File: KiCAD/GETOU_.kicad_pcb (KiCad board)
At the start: 2 copper layers, 109.5 x 59.5 mm, 25 parts, among them U1 XIAO-RP2040-DIP

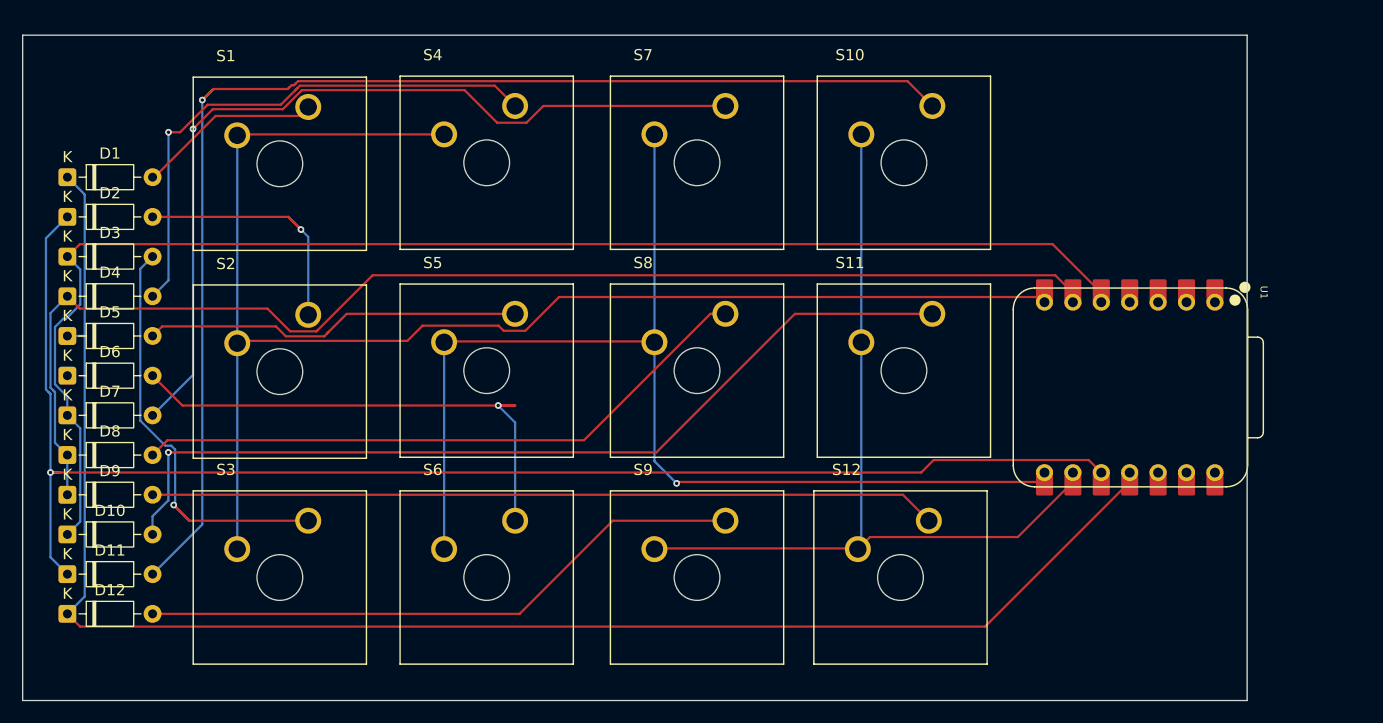
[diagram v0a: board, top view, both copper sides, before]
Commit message: Add stuff
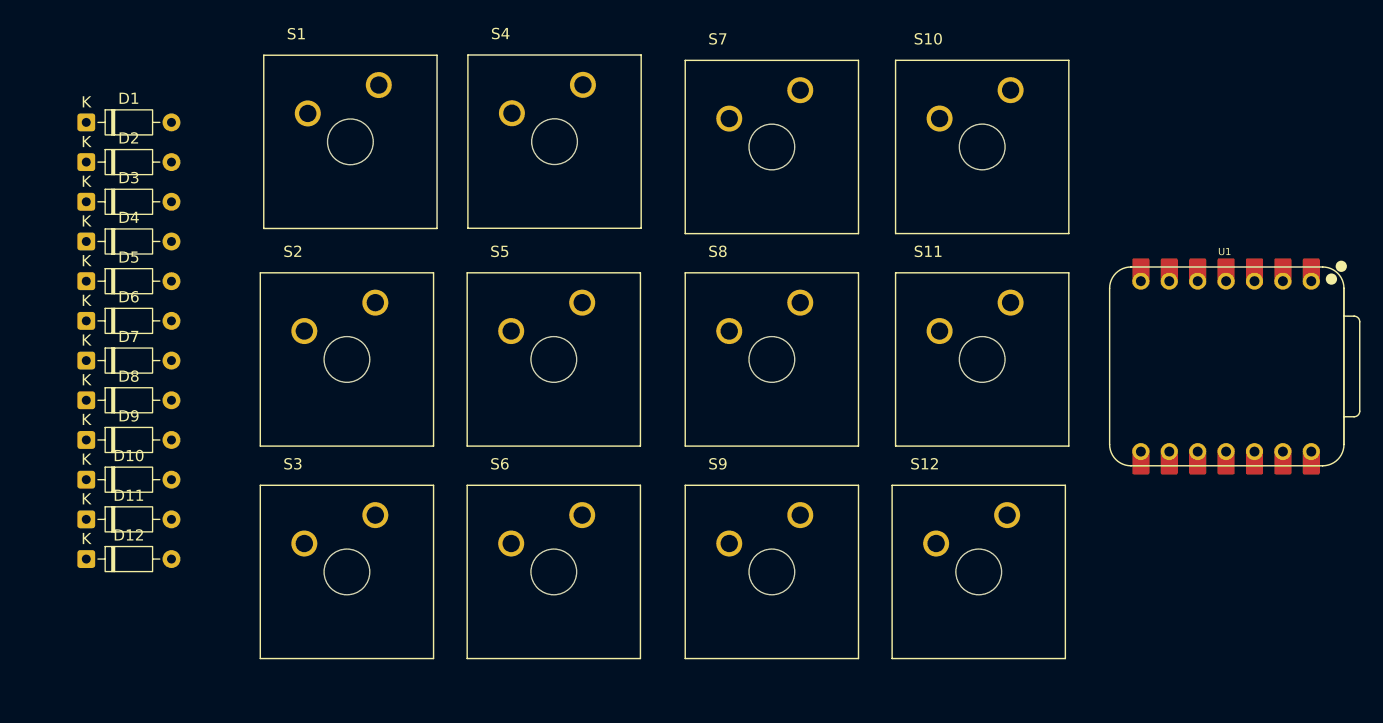
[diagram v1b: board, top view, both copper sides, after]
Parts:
- moved U1 8.82 mm to (199.6, 91.6), turned to 0 degrees
- moved S10 7.14 mm to (177.8, 72.0)
- moved S11 7.07 mm to (177.8, 91.0)
- moved S12 7.02 mm to (177.5, 110.0)
- moved S7 6.84 mm to (159.0, 72.0)
- moved S8 6.76 mm to (159.0, 91.0)
- moved S9 6.71 mm to (159.0, 110.0)
- moved S1 6.61 mm to (121.3, 71.5)
- moved S4 6.35 mm to (139.6, 71.5)
- moved S2 6.10 mm to (121.0, 91.0)
- moved S5 6.08 mm to (139.5, 91.0)
- moved S3 6.02 mm to (121.0, 110.0)
- moved S6 6.02 mm to (139.5, 110.0)
- moved D1 5.18 mm to (97.7, 69.8)
- moved D10 5.18 mm to (97.7, 101.8)
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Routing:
- net col0: track 143.5 -> 0.00 mm
- net col1: track 131.3 -> 0.00 mm, vias 1 -> 0
- net row0: track 130.7 -> 0.00 mm
- net col2: track 123.4 -> 0.00 mm
- net Net-(D11-A): track 114.3 -> 0.00 mm, vias 1 -> 0
- net col3: track 114.2 -> 0.00 mm
- net row1: track 103.2 -> 0.00 mm, vias 1 -> 0
- net Net-(D10-A): track 81.4 -> 0.00 mm, vias 1 -> 0
- net Net-(D7-A): track 79.3 -> 0.00 mm, vias 1 -> 0
- net row2: track 78.0 -> 0.00 mm
- net Net-(D9-A): track 70.4 -> 0.00 mm
- net Net-(D8-A): track 56.5 -> 0.00 mm
- net Net-(D12-A): track 54.7 -> 0.00 mm
- net Net-(D6-A): track 49.0 -> 0.00 mm, vias 1 -> 0
- net Net-(D4-A): track 49.0 -> 0.00 mm, vias 1 -> 0
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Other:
- board outline removed
